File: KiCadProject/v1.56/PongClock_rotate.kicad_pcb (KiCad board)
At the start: 2 copper layers, 88.9 x 67.3 mm, 24 parts, among them J1 CONN_01X01_MALE, J2 MY_USB_OTG, SW1 SW_DIP_x02, SW2 SW_DIP_x02, U1 TinyRTC_I2C_RIGHT, U2 MAX7219_IN, U3 MAX7219_IN, U4 MAX7219_IN, U5 MAX7219_IN, U6 MAX7219_IN, U7 MAX7219_IN, U8 ATMEGA328P-PU, U9 FTDI1232, Y1 Crystal

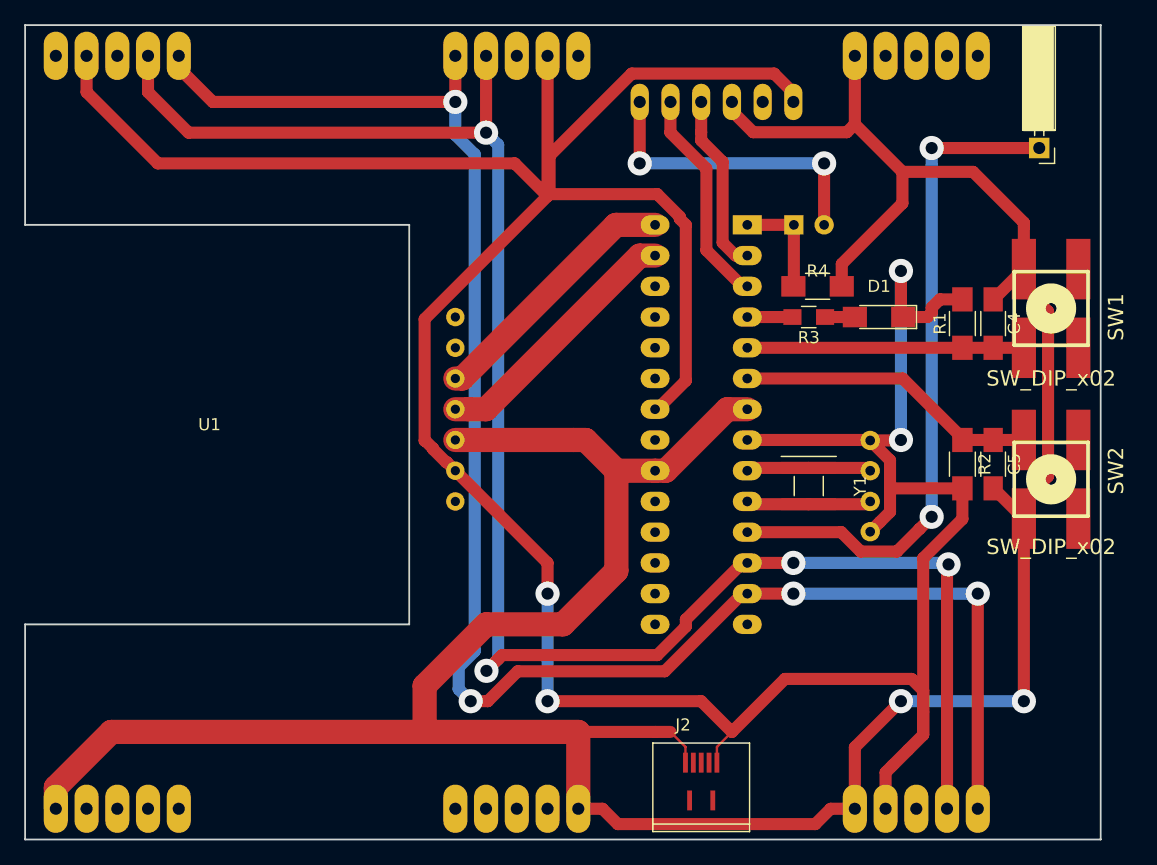
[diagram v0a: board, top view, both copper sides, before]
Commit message: v1.56
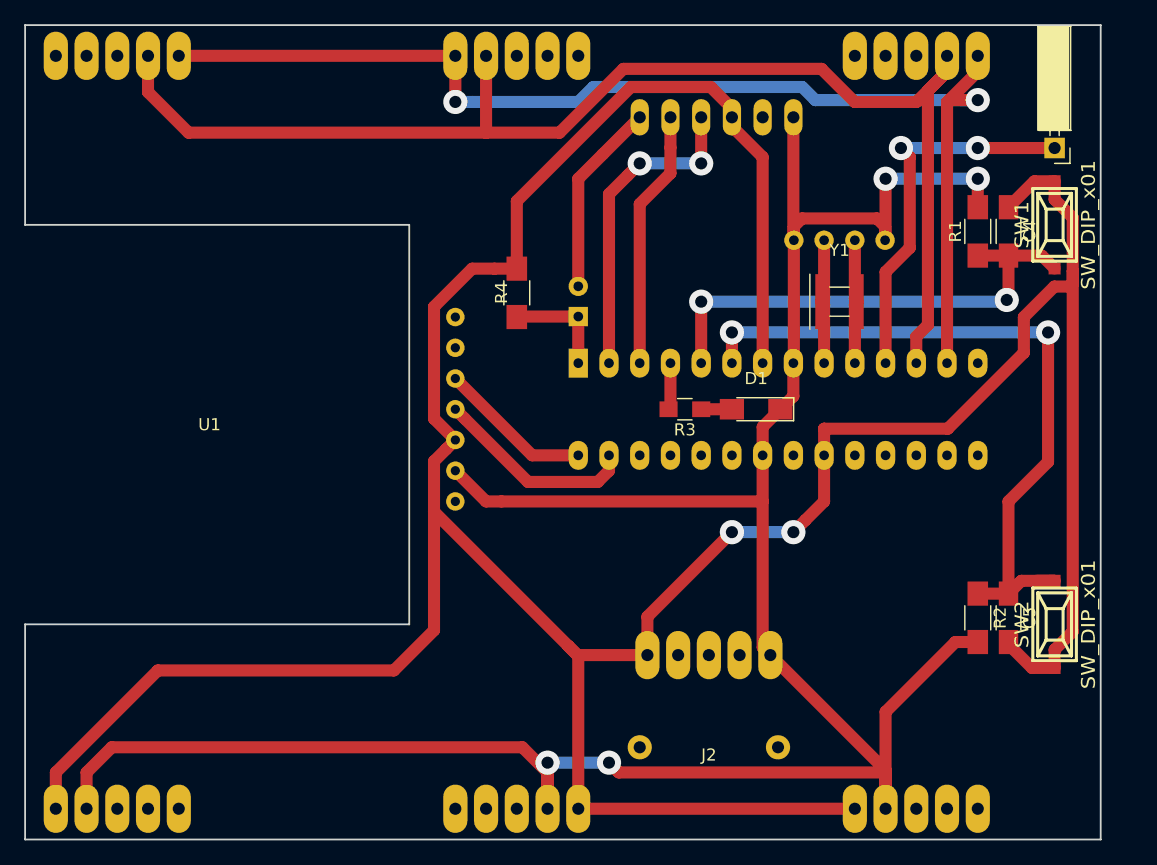
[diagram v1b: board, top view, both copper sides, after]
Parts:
- J2: footprint Connectors:USB_Micro-B_10103594-0001LF -> PongClock:USB_BOARD
- SW1, SW2: value SW_DIP_x02 -> SW_DIP_x01; footprint PongClock:PCB_PUSH_POOR_SMD -> mod_switch:smd_push
- moved R4 24.9 mm to (142.2, 72.9), turned to 270 degrees
- moved C2 21.6 mm to (170.2, 68.6), turned to 0 degrees
- moved C1 19.4 mm to (167.6, 68.6), turned to 180 degrees
- moved C3 19.4 mm to (147.3, 74.9), turned to 90 degrees
- moved U8 18.1 mm to (147.3, 78.7), turned to 270 degrees
- moved Y1 15.5 mm to (168.9, 73.7), turned to 0 degrees
- moved R3 12.8 mm to (156.1, 82.5)
- moved R2 12.8 mm to (180.3, 99.8)
- moved C5 12.8 mm to (182.9, 99.8)
- moved D1 12.7 mm to (162.0, 82.5)
- moved SW2 12.0 mm to (186.7, 100.3), turned to 90 degrees
- moved J2 10.8 mm to (168.3, 113.0), turned to 180 degrees
- moved R1 7.73 mm to (180.3, 67.8)
- moved C4 7.73 mm to (182.9, 67.8)
- moved SW1 6.91 mm to (186.7, 67.3), turned to 90 degrees
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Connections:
- net Net-(C3-Pad2) renamed DTR
- SW1 pad 2: (no net) -> VCC
- SW2 pad 2: (no net) -> SW2
- U2 pad 2: (no net) -> GND
- U3 pad 2: (no net) -> GND
- U4 pad 4: LATCH -> (no net)
- U4 pad 5: CLK -> (no net)
- U5 pad 2: GND -> (no net)
- U6 pad 2: GND -> (no net)
- U7 pad 1: VCC -> (no net)
- U7 pad 4: (no net) -> LATCH
- U7 pad 5: (no net) -> CLK
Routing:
- net GND: track 285.9 -> 213.2 mm
- net CLK: track 143.4 -> 101.3 mm, vias 4 -> 2
- net LATCH: track 146.5 -> 107.6 mm, vias 4 -> 0
- net SW2: track 25.1 -> 59.9 mm, vias 0 -> 2
- net VCC: track 265.9 -> 291.8 mm
- net MAX_IN: track 56.5 -> 31.6 mm
- net SW1: track 22.9 -> 40.9 mm, vias 0 -> 2
- net RX: track 14.8 -> 26.5 mm, vias 0 -> 2
- net DTR: track 25.4 -> 16.1 mm, vias 2 -> 0
- net SCL: track 21.8 -> 12.8 mm
- net SDA: track 21.8 -> 16.8 mm
- net TX: track 18.1 -> 21.4 mm
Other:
- net class Default: clearance 0.34 -> 0.5; trace_width 2 -> 1
- rule trace_clearance: 0.34 -> 0.5
- rule trace_min: 0.2 -> 0.5
- board text added: "PongClock v1.56"
- board text removed: "PongClock v1.55"
